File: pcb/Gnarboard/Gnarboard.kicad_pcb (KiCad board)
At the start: 2 copper layers, 155 x 130 mm, 134 parts, among them J1 N2K, J10 Screw_Terminal_01x02, J11 Screw_Terminal_01x02, J12 Screw_Terminal_01x02, J2 I2C, J3 Screw_Terminal_01x12, J4 Screw_Terminal_01x12, J5 Screw_Terminal_01x02, J6 Screw_Terminal_01x02, J7 Screw_Terminal_01x02, J8 Screw_Terminal_01x02, J9 Screw_Terminal_01x02, Q1 BC817, Q10 IRF4905, Q11 BC817, Q12 IRF4905, Q13 BC817, Q14 IRF4905, Q15 BC817, Q16 IRF4905, Q2 IRF4905, Q3 BC817, Q4 IRF4905, Q5 BC817, Q6 IRF4905, Q7 BC817, Q8 IRF4905, Q9 BC817, U1 ESP32-DEVKITC, U10 ACS725xLCTR-20AU, U11 ACS725xLCTR-20AU, U12 ACS725xLCTR-20AU, U2 MCP3208, U4 D24V5F3, U5 ACS725xLCTR-20AU, U6 ACS725xLCTR-20AU, U7 ACS725xLCTR-20AU, U8 ACS725xLCTR-20AU, U9 ACS725xLCTR-20AU

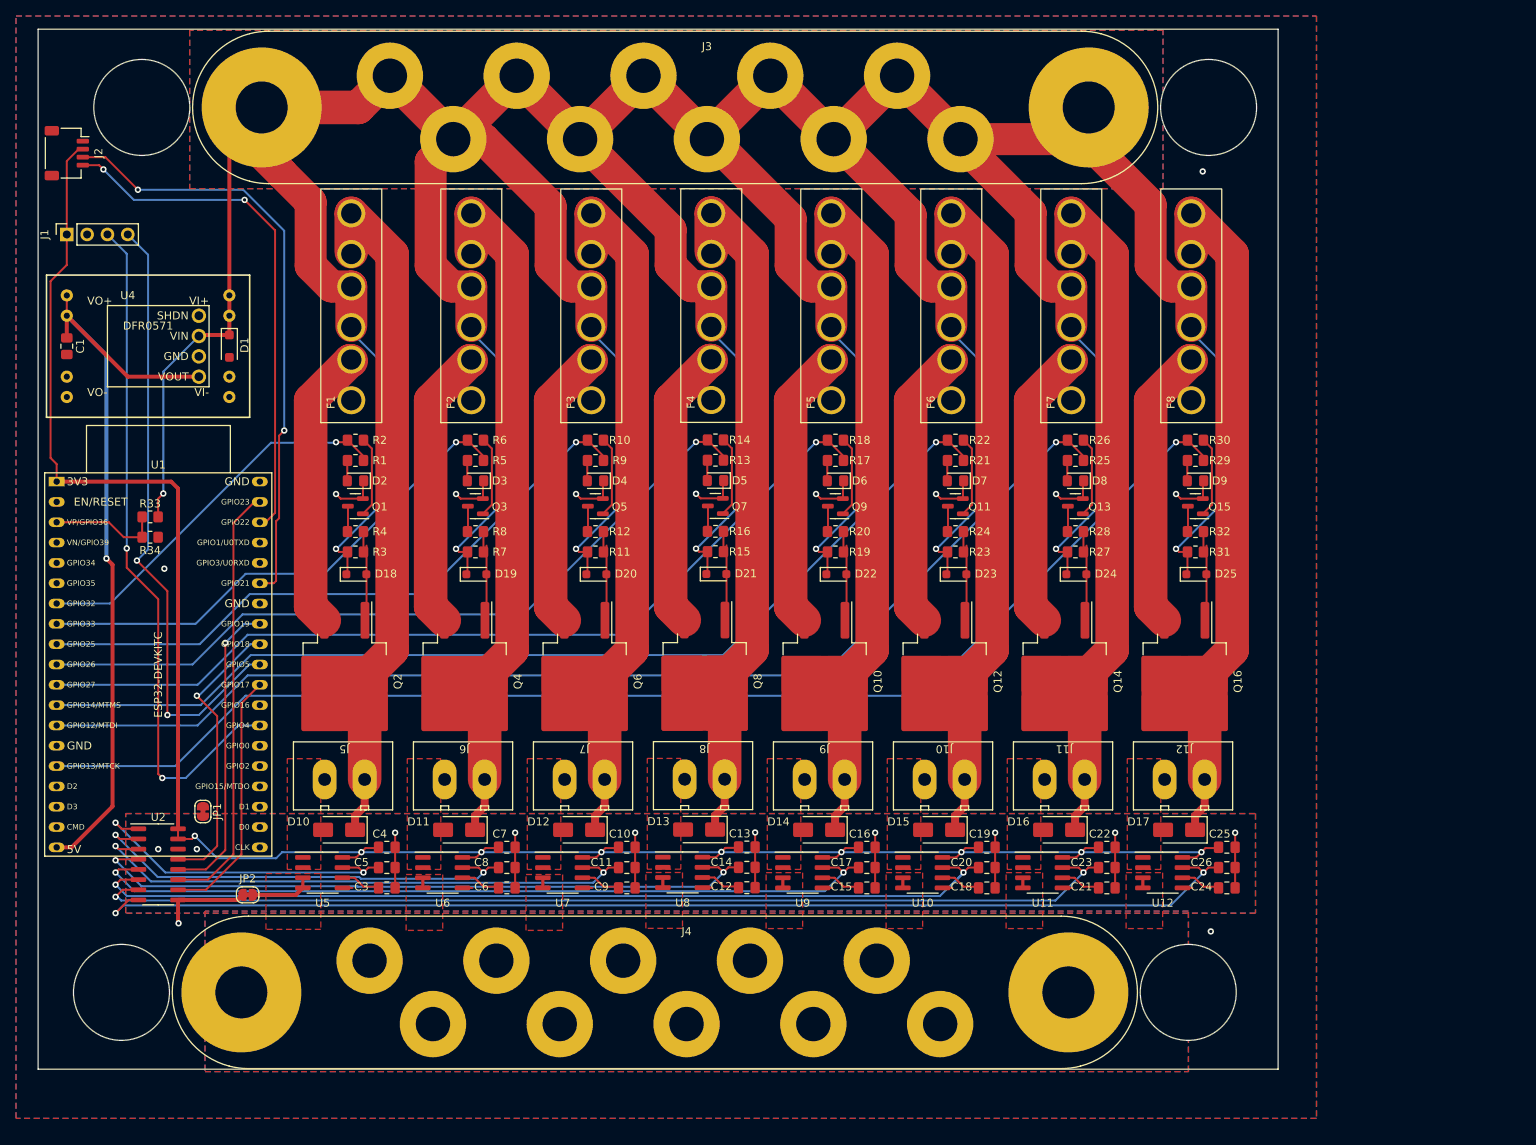
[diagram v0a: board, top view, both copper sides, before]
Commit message: pcb stuff
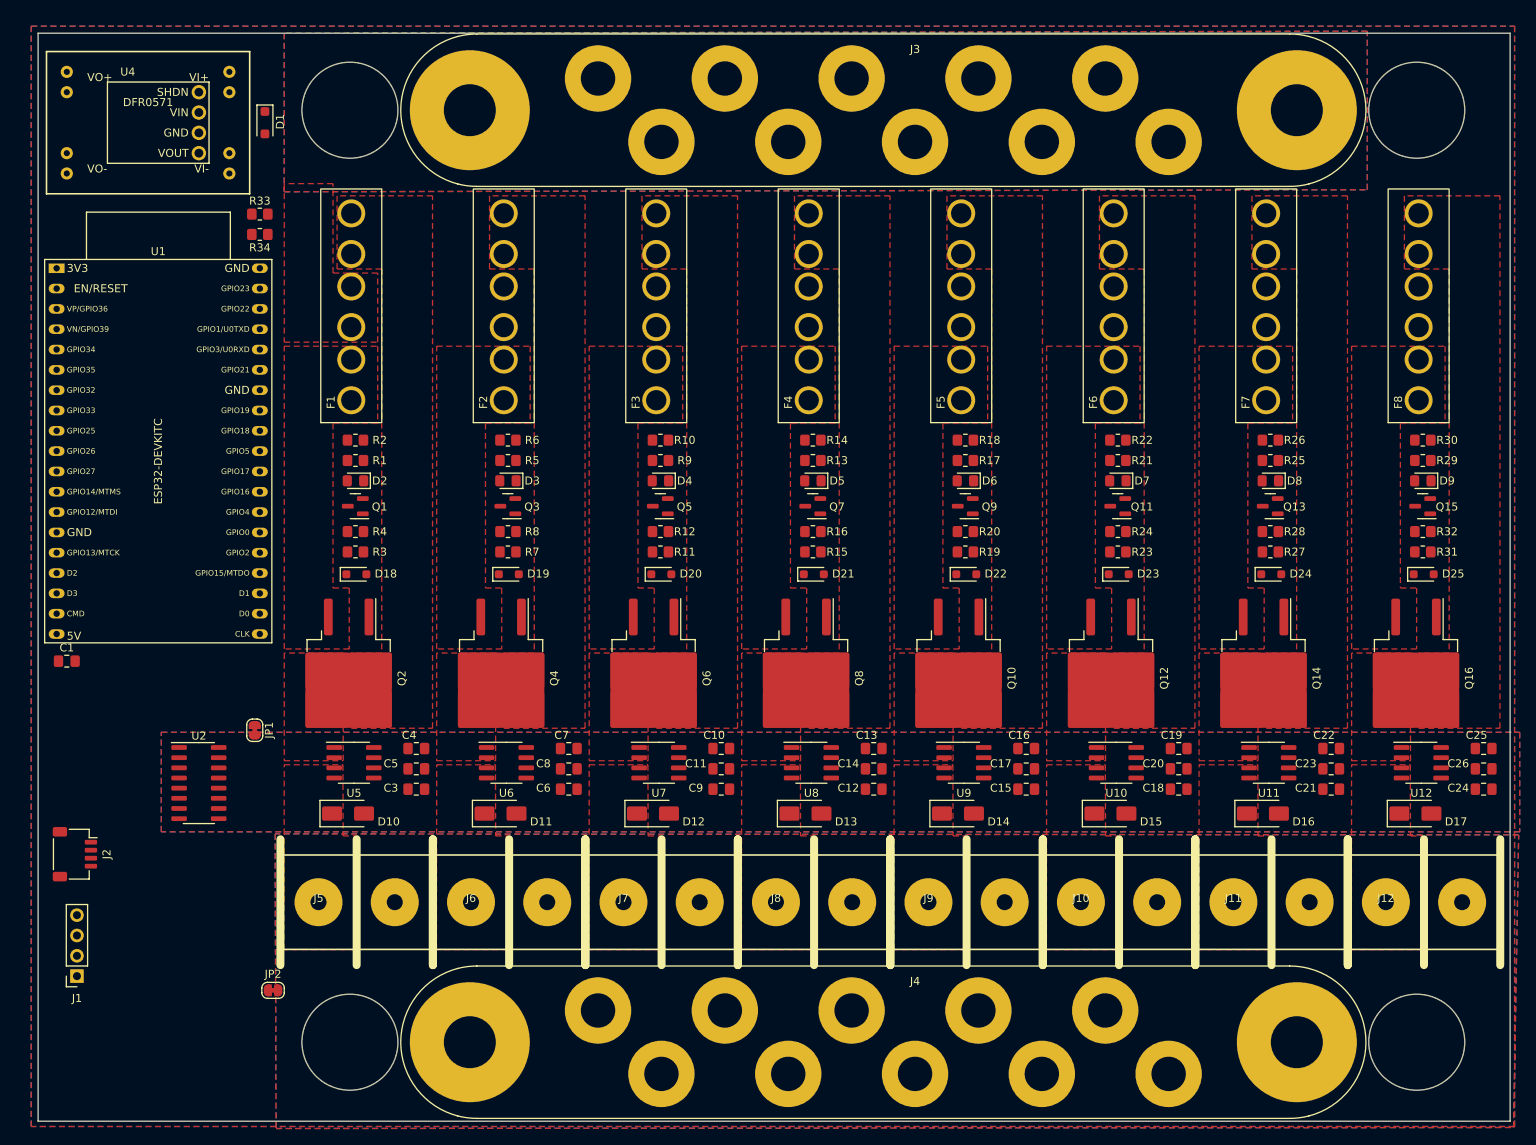
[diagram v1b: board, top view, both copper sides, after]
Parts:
- D10, D11, D12, D13, D14, D15, D16, D17: value GS1G-LTP -> SS16
- J10, J11, J12, J5, J6, J7, J8, J9: footprint gnarboard:Amphenol OQ02715 -> gnarboard:Molex 1x02 .375
- R11, R15, R19, R23, R27, R3, R31, R7: value 33k -> 22k
- R12, R16, R20, R24, R28, R32, R4, R8: value 6.8k -> 4.7k
- moved J1 92.7 mm to (66.0, 142.2), turned to 180 degrees
- moved J2 87.6 mm to (65.8, 127.0)
- moved R34 40.3 mm to (88.9, 49.5)
- moved R33 40.3 mm to (88.9, 47.0)
- moved C1 39.4 mm to (64.8, 102.9), turned to 0 degrees
- moved U12 35.1 mm to (234.1, 115.6)
- moved C26 34.4 mm to (241.9, 116.3)
- moved C24 34.4 mm to (241.9, 118.9)
- moved C25 34.4 mm to (241.9, 113.8)
- moved J12 33.6 mm to (234.4, 133.0), turned to 0 degrees
- moved U11 31.4 mm to (215.0, 115.6)
- moved C21 30.6 mm to (222.8, 118.9)
- moved C23 30.6 mm to (222.8, 116.3)
- moved C22 30.6 mm to (222.8, 113.8)
- moved J11 30.1 mm to (215.4, 133.0), turned to 0 degrees
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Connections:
- D10 pad 2: Net-(D10-A) -> GNDPWR
- D11 pad 2: Net-(D11-A) -> GNDPWR
- D12 pad 2: Net-(D12-A) -> GNDPWR
- D13 pad 2: Net-(D13-A) -> GNDPWR
- D14 pad 2: Net-(D14-A) -> GNDPWR
- D15 pad 2: Net-(D15-A) -> GNDPWR
- D16 pad 2: Net-(D16-A) -> GNDPWR
- D17 pad 2: Net-(D17-A) -> GNDPWR
- F1 pad 3: Net-(D10-K) -> Net-(Q2-D)
- F2 pad 3: Net-(D11-K) -> Net-(Q4-D)
- F3 pad 3: Net-(D12-K) -> Net-(Q6-D)
- F4 pad 3: Net-(D13-K) -> Net-(Q8-D)
- F5 pad 3: Net-(D14-K) -> Net-(Q10-D)
- F6 pad 3: Net-(D15-K) -> Net-(Q12-D)
- F7 pad 3: Net-(D16-K) -> Net-(Q14-D)
- F8 pad 3: Net-(D17-K) -> Net-(Q16-D)
- J10 pad 2: Net-(D15-A) -> GNDPWR
- J11 pad 2: Net-(D16-A) -> GNDPWR
- J12 pad 2: Net-(D17-A) -> GNDPWR
- J5 pad 2: Net-(D10-A) -> GNDPWR
- J6 pad 2: Net-(D11-A) -> GNDPWR
- J7 pad 2: Net-(D12-A) -> GNDPWR
- J8 pad 2: Net-(D13-A) -> GNDPWR
- J9 pad 2: Net-(D14-A) -> GNDPWR
- Q10 pad 2: Net-(D14-K) -> Net-(Q10-D)
- Q12 pad 2: Net-(D15-K) -> Net-(Q12-D)
- Q14 pad 2: Net-(D16-K) -> Net-(Q14-D)
- Q16 pad 2: Net-(D17-K) -> Net-(Q16-D)
- Q2 pad 2: Net-(D10-K) -> Net-(Q2-D)
- Q4 pad 2: Net-(D11-K) -> Net-(Q4-D)
- Q6 pad 2: Net-(D12-K) -> Net-(Q6-D)
- Q8 pad 2: Net-(D13-K) -> Net-(Q8-D)
- U10 pad 1: Net-(D15-A) -> Net-(Q12-D)
- U10 pad 2: Net-(D15-A) -> Net-(Q12-D)
- U10 pad 3: GNDPWR -> Net-(D15-K)
- U10 pad 4: GNDPWR -> Net-(D15-K)
- U11 pad 1: Net-(D16-A) -> Net-(Q14-D)
- U11 pad 2: Net-(D16-A) -> Net-(Q14-D)
- U11 pad 3: GNDPWR -> Net-(D16-K)
- U11 pad 4: GNDPWR -> Net-(D16-K)
- U12 pad 1: Net-(D17-A) -> Net-(Q16-D)
- U12 pad 2: Net-(D17-A) -> Net-(Q16-D)
- U12 pad 3: GNDPWR -> Net-(D17-K)
- U12 pad 4: GNDPWR -> Net-(D17-K)
- U5 pad 1: Net-(D10-A) -> Net-(Q2-D)
- U5 pad 2: Net-(D10-A) -> Net-(Q2-D)
- U5 pad 3: GNDPWR -> Net-(D10-K)
- U5 pad 4: GNDPWR -> Net-(D10-K)
- U6 pad 1: Net-(D11-A) -> Net-(Q4-D)
- U6 pad 2: Net-(D11-A) -> Net-(Q4-D)
- U6 pad 3: GNDPWR -> Net-(D11-K)
- U6 pad 4: GNDPWR -> Net-(D11-K)
- U7 pad 1: Net-(D12-A) -> Net-(Q6-D)
- U7 pad 2: Net-(D12-A) -> Net-(Q6-D)
- U7 pad 3: GNDPWR -> Net-(D12-K)
- U7 pad 4: GNDPWR -> Net-(D12-K)
- U8 pad 1: Net-(D13-A) -> Net-(Q8-D)
- U8 pad 2: Net-(D13-A) -> Net-(Q8-D)
- U8 pad 3: GNDPWR -> Net-(D13-K)
- U8 pad 4: GNDPWR -> Net-(D13-K)
- U9 pad 1: Net-(D14-A) -> Net-(Q10-D)
- U9 pad 2: Net-(D14-A) -> Net-(Q10-D)
- U9 pad 3: GNDPWR -> Net-(D14-K)
- U9 pad 4: GNDPWR -> Net-(D14-K)
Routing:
- net +24V: track 733.6 -> 0.00 mm, vias 9 -> 0
- net +3.3V: track 271.9 -> 0.00 mm, vias 9 -> 0
- net /PWM7: track 161.1 -> 0.00 mm, vias 1 -> 0
- net /ADC7: track 146.7 -> 0.00 mm, vias 2 -> 0
- net /PWM6: track 144.0 -> 0.00 mm, vias 1 -> 0
- net /ADC6: track 131.0 -> 0.00 mm, vias 2 -> 0
- net /PWM5: track 127.9 -> 0.00 mm, vias 1 -> 0
- net /ADC5: track 118.8 -> 0.00 mm, vias 2 -> 0
- net /PWM4: track 111.8 -> 0.00 mm, vias 1 -> 0
- net /ADC4: track 101.0 -> 0.00 mm, vias 2 -> 0
- net +5V: track 97.8 -> 0.00 mm, vias 1 -> 0
- net /PWM3: track 95.8 -> 0.00 mm, vias 1 -> 0
- net /ADC3: track 86.1 -> 0.00 mm, vias 2 -> 0
- net CAN_RX: track 86.0 -> 0.00 mm, vias 2 -> 0
- net Net-(D11-K): track 84.4 -> 0.00 mm
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- added copper zone on F.Cu, net Net-(D10-K)
- added copper zone on F.Cu, net Net-(D11-K)
- added copper zone on F.Cu, net Net-(D12-K)
- added copper zone on F.Cu, net Net-(D13-K)
- added copper zone on F.Cu, net Net-(D14-K)
- added copper zone on F.Cu, net Net-(D15-K)
- added copper zone on F.Cu, net Net-(D16-K)
- added copper zone on F.Cu, net Net-(D17-K)
- added copper zone on F.Cu, net Net-(Q10-D)
- added copper zone on F.Cu, net Net-(Q10-S)
- added copper zone on F.Cu, net Net-(Q12-D)
- added copper zone on F.Cu, net Net-(Q12-S)
- added copper zone on F.Cu, net Net-(Q14-D)
- added copper zone on F.Cu, net Net-(Q14-S)
- added copper zone on F.Cu, net Net-(Q16-D)
- added copper zone on F.Cu, net Net-(Q16-S)
- added copper zone on F.Cu, net Net-(Q2-D)
- added copper zone on F.Cu, net Net-(Q2-S)
- added copper zone on F.Cu, net Net-(Q4-D)
- added copper zone on F.Cu, net Net-(Q4-S)
- added copper zone on F.Cu, net Net-(Q6-D)
- added copper zone on F.Cu, net Net-(Q6-S)
- added copper zone on F.Cu, net Net-(Q8-D)
- added copper zone on F.Cu, net Net-(Q8-S)
- removed copper zone on F.Cu, net Net-(D10-A)
- removed copper zone on F.Cu, net Net-(D11-A)
- removed copper zone on F.Cu, net Net-(D12-A)
- removed copper zone on F.Cu, net Net-(D13-A)
- removed copper zone on F.Cu, net Net-(D14-A)
- removed copper zone on F.Cu, net Net-(D15-A)
- removed copper zone on F.Cu, net Net-(D16-A)
- removed copper zone on F.Cu, net Net-(D17-A)
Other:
- board size 155 x 130 mm -> 184 x 136 mm
